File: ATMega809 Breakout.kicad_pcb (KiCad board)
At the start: 2 copper layers, 77.9 x 41.4 mm, 51 parts, among them J1 USB_B_Micro, J2 Conn_01x05, J3 Conn_01x20, J4 Conn_01x12, J5 UPDI, Q1 PJA3438-AU, Q2 PJA3438-AU, Q3 PJA3438-AU, Q4 PJA3438-AU, Q5 PJA3438-AU, SW1 RESET, U1 NCP1117-ADJ_SOT223, U2 ATMEGA809-AF

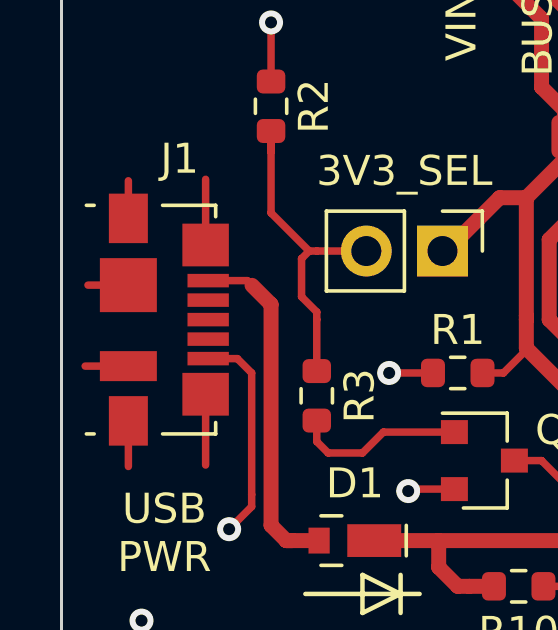
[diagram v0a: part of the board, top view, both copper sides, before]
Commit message: Final tweaks and checks.
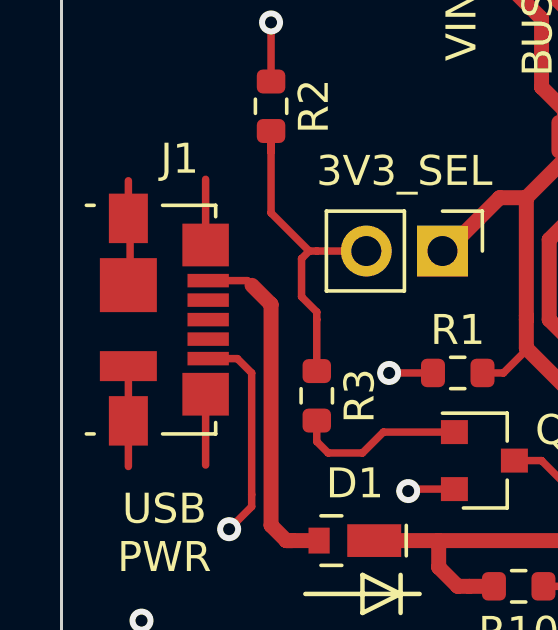
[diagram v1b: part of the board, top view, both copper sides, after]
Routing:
- net GND: track 95.8 -> 97.3 mm
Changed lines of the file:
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@@
     (thickness 1.6)
     (drawings 89)
-    (tracks 680)
+    (tracks 682)
     (zones 0)
     (modules 51)
@@
   (segment (start 105.134 45.7725) (end 105.134 43.583) (width 0.25) (layer F.Cu) (net 1))
   (segment (start 102.559 44.885) (end 102.559 43.631) (width 0.25) (layer F.Cu) (net 1))
-  (segment (start 102.559 47.11) (end 101.212 47.11) (width 0.25) (layer F.Cu) (net 1))
-  (segment (start 102.559 49.81) (end 101.118 49.81) (width 0.25) (layer F.Cu) (net 1))
   (via (at 135.509 57.15) (size 0.8) (drill 0.4) (layers F.Cu B.Cu) (net 1))
   (segment (start 129.921 48.387) (end 130.365 47.943) (width 0.25) (layer F.Cu) (net 1))
@@
   (via (at 173.736 60.452) (size 0.8) (drill 0.4) (layers F.Cu B.Cu) (net 1))
   (via (at 166.37 66.802) (size 0.8) (drill 0.4) (layers F.Cu B.Cu) (net 1))
+  (segment (start 102.559 51.635) (end 102.559 49.968) (width 0.25) (layer F.Cu) (net 1))
+  (segment (start 102.559 47.11) (end 102.496 47.11) (width 0.25) (layer F.Cu) (net 1))
+  (segment (start 102.496 47.11) (end 102.616 46.99) (width 0.25) (layer F.Cu) (net 1))
+  (segment (start 102.616 46.99) (end 102.616 44.577) (width 0.25) (layer F.Cu) (net 1))
   (segment (start 118.696 52.084) (end 115.824 49.212) (width 0.5) (layer F.Cu) (net 2))
   (segment (start 119.659 52.084) (end 118.696 52.084) (width 0.5) (layer F.Cu) (net 2))
